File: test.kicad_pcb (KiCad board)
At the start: 2 copper layers, 161 parts, among them Q1 T2N7002AK, Q2 T2N7002AK, SW1 SW_Push, U1 ESP32-S3-WROOM-1, U2 LD1117S33TR_SOT223, U3 SN75176AD, U4 LM321, U5 LM321

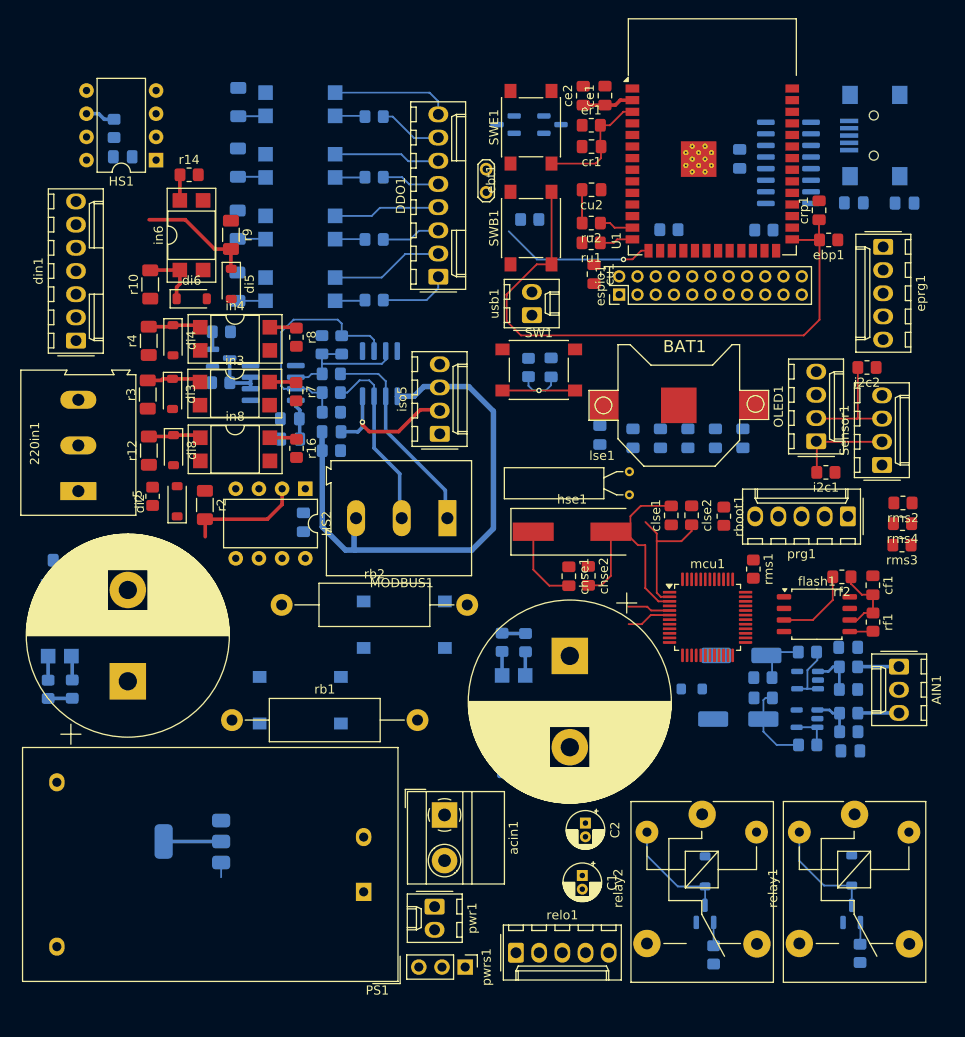
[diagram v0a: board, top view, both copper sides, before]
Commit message: final placement-no route
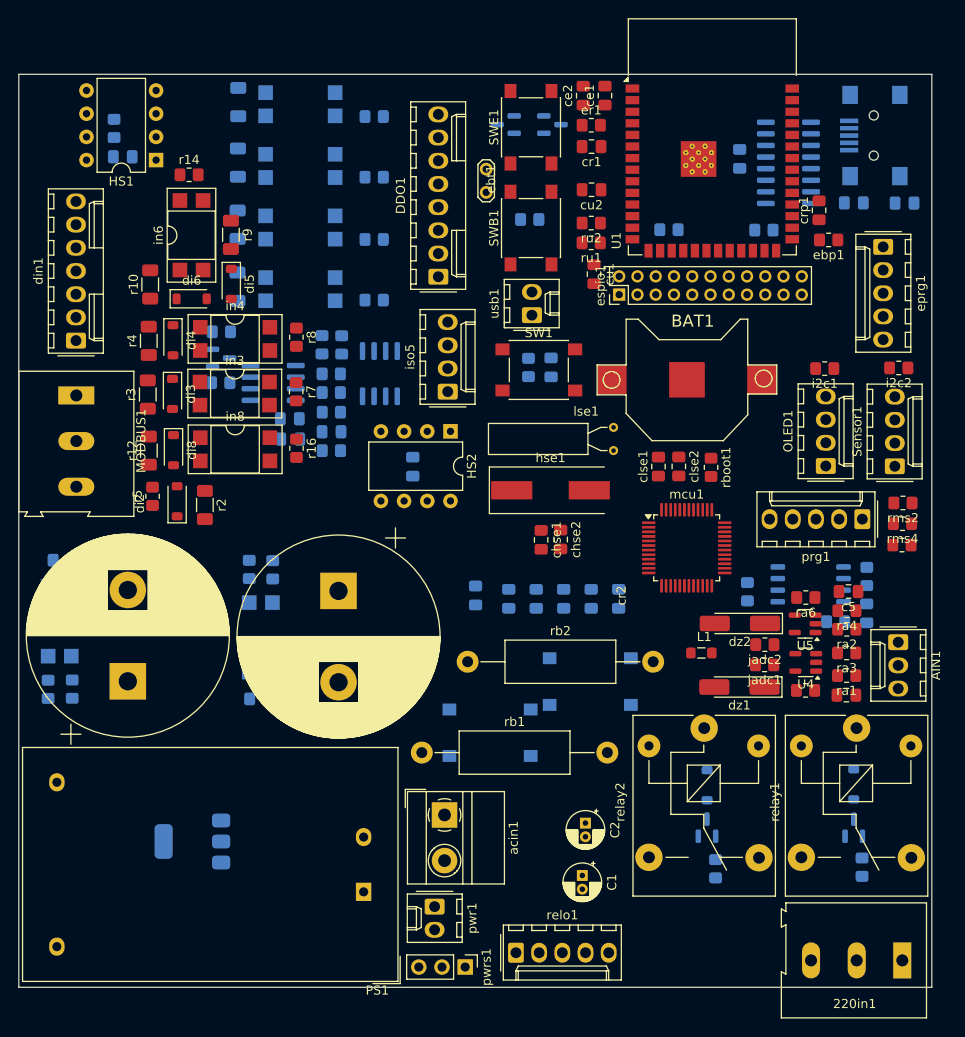
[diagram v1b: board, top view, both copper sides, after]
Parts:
- L1, U4, U5, c4, c5, dz1, dz2, jadc1, jadc2, ra1, ra2, ra3, ra4, ra5, ra6: moved to F.Cu
- cf1, flash1, rf1, rf2, rms1: moved to B.Cu
- moved 220in1 103.9 mm to (96.8, 97.0), turned to 180 degrees
- moved MODBUS1 42.8 mm to (6.30, 35.2), turned to -90 degrees
- moved aco2 28.8 mm to (26.5, 61.7)
- moved r18 28.8 mm to (27.8, 54.3)
- moved r20 28.8 mm to (25.2, 54.2)
- moved r22 28.8 mm to (26.3, 68.4)
- moved cr2 26.3 mm to (35.0, 56.6)
- moved cb1 22.2 mm to (50.0, 57.1)
- moved cm3 22.2 mm to (59.7, 57.4)
- moved cm1 22.2 mm to (65.7, 57.4)
- moved cm2 22.2 mm to (62.7, 57.4)
- moved cm4 22.2 mm to (56.7, 57.4)
- moved cm5 22.2 mm to (53.7, 57.4)
- moved bridge2 21.3 mm to (62.6, 66.5)
- moved rb2 21.3 mm to (49.2, 64.3)
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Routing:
- net /ESP_GPIO_0: track 66.8 -> 0.00 mm
- net MGND: track 59.4 -> 0.00 mm
- net /RS485_B: track 26.5 -> 0.00 mm
- net /RS485_AO: track 23.2 -> 0.00 mm
- net /+3.3V: track 20.4 -> 0.00 mm
- net /RS485_BO: track 20.4 -> 0.00 mm
- net Net-(mcu1-PC14): track 17.2 -> 0.00 mm
- net Net-(U1-IO3): track 17.0 -> 0.00 mm, vias 1 -> 0
- net /+M5V: track 16.6 -> 0.00 mm, vias 1 -> 0
- net /RS485_A: track 15.5 -> 0.00 mm
- net Net-(mcu1-PC13): track 14.8 -> 0.00 mm
- net Net-(mcu1-PF1): track 13.8 -> 0.00 mm
- net /ESP_EN: track 13.4 -> 0.00 mm
- net /DO4: track 13.2 -> 0.00 mm
- net /RESET: track 12.9 -> 0.00 mm, vias 1 -> 0
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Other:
- board outline added: 100 x 100 mm
